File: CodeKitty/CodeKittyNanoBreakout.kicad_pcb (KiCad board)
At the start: 2 copper layers, 17.8 x 43.2 mm, 11 parts, among them P1 CONN_01X02, P2 CONN_01X02, P3 CONN_01X03, P4 CONN_01X03, P5 CONN_01X02, U1 ArduinoNano

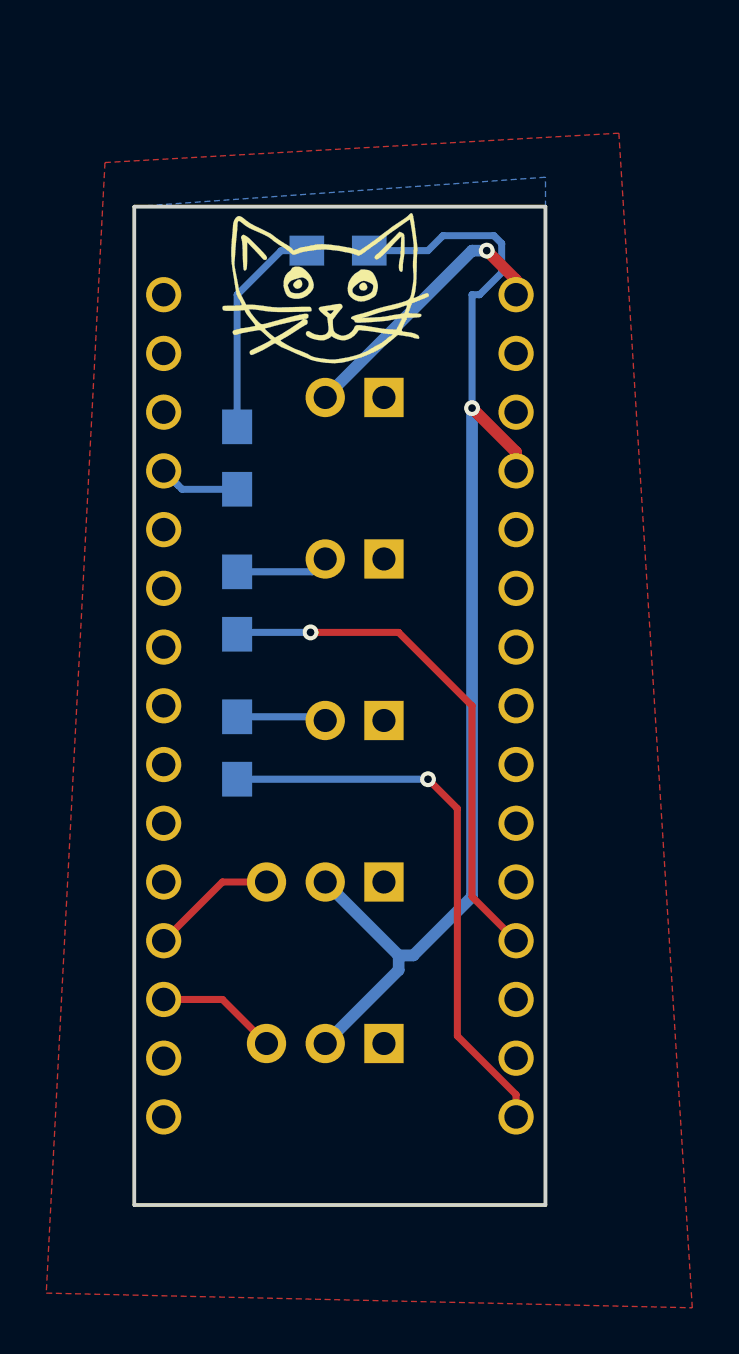
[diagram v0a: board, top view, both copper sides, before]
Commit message: update of codekitty
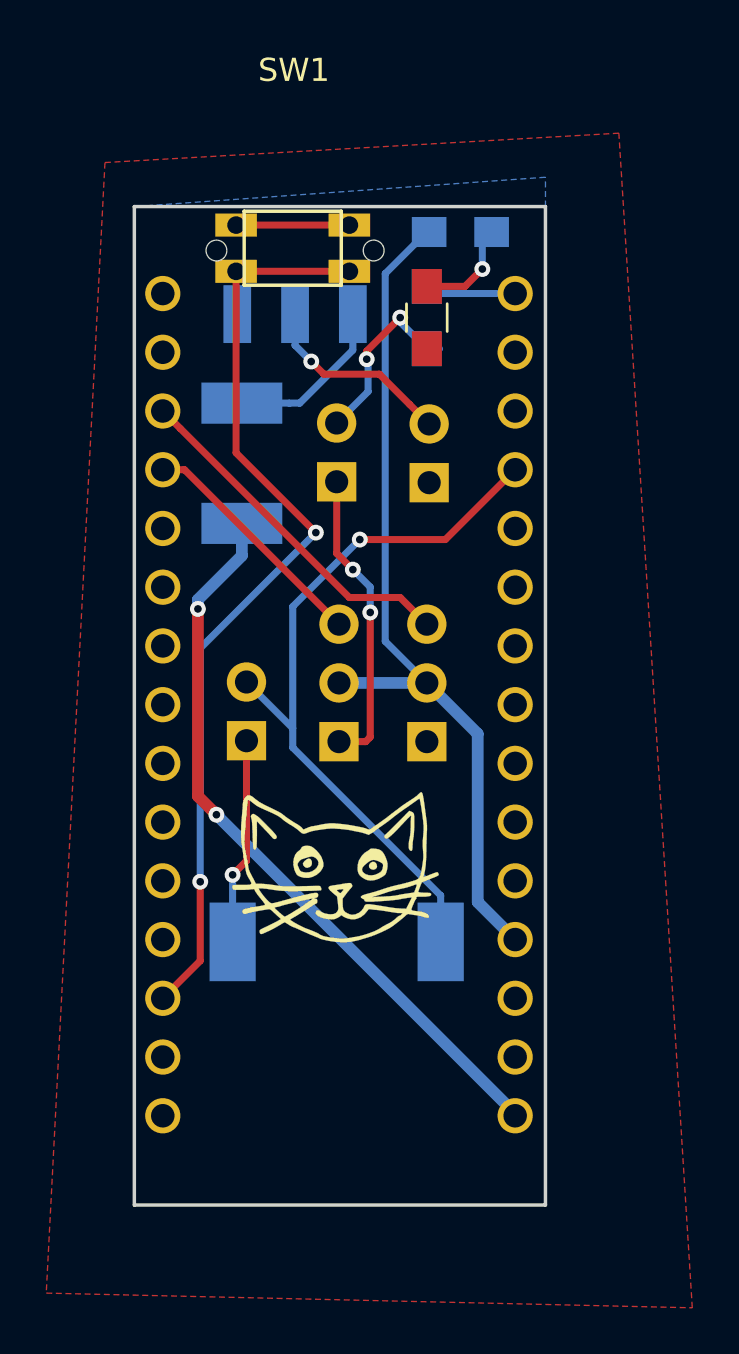
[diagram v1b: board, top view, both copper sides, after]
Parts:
- removed R3: R, Resistors_SMD:R_0805_HandSoldering
- added F1: F_Small, DM_Custom:DM_FUSE_PTC0ZCG, B.Cu at (201.5, 93.7)
- added SP1: SPEAKER, DM_Custom:DM_PiezSMD_PMKCS0909E4000-R1, B.Cu at (205.6, 114.3)
- added SW1: SW_PUSH_SMALL_H, DM_Custom:DM_SMD_BUTTON_PTS810, F.Cu at (203.7, 84.3)
- added SW2: Switch_SPDT_x2, DM_Custom:DM_SPDT_RTAngle_JS102011SAQN, B.Cu at (203.8, 84.5)
- R1: moved to F.Cu
- U1: moved to B.Cu
- moved G*** 25.0 mm to (205.4, 111.2)
- moved R2 20.3 mm to (209.5, 87.3), turned to 90 degrees
- moved P4 13.2 mm to (209.5, 105.7), turned to 0 degrees
- moved P2 10.5 mm to (205.6, 94.5), turned to 0 degrees
- moved R1 10.2 mm to (209.5, 87.3)
- moved P5 9.86 mm to (201.7, 105.7), turned to 0 degrees
- moved P3 6.37 mm to (205.7, 105.7), turned to 0 degrees
- moved D1 5.35 mm to (210.9, 83.7), turned to 180 degrees
- moved P1 4.17 mm to (209.6, 94.5), turned to 0 degrees
- moved U1 0.06 mm to (205.7, 104.1)
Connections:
- P1 pad 2: VCC -> Net-(P1-Pad2)
- P5 pad 2: Net-(P5-Pad2) -> BUZZ
- U1 pad 3: Net-(U1-Pad3) -> RST
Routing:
- net RST: track 0.00 -> 40.5 mm, vias 0 -> 2
- net GND: track 4.40 -> 26.9 mm, vias 0 -> 3
- net TAIL: track 24.4 -> 3.95 mm, vias 1 -> 0
- net VCC: track 12.0 -> 32.1 mm, vias 1 -> 2
- net 5V: track 52.5 -> 37.6 mm, vias 1 -> 0
- net RSERVO: track 5.23 -> 15.2 mm
- net BUZZ: track 22.5 -> 32.1 mm
- net Net-(P1-Pad2): track 0.00 -> 8.56 mm, vias 0 -> 1
- net Net-(F1-Pad1): track 0.00 -> 7.31 mm
- net Net-(D1-Pad1): track 9.52 -> 4.48 mm, vias 0 -> 1
- net LSERVO: track 5.50 -> 10.4 mm
- net Net-(P2-Pad2): track 3.88 -> 8.13 mm, vias 0 -> 2
- net Net-(P5-Pad2): track 4.04 -> 0.00 mm
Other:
- board text added: "CodeKitty DM100917"
- board text removed: "CodeKitty DM073117"
